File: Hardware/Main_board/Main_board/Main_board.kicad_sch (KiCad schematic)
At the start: 73 parts, among them J2 Conn_01x03_Pin, J3 B9B-XH-A(LF)(SN), J4 282814-2, J5 282814-2, J6 B8B-XH-A(LF)(SN), J6 Power 5V, J7 Power 3v3, J8 GND, J9 Button 1, Q1 2SC1815, U1 L7805, U13 LM358DT, U14 74HC14D, U15 74HC14D, U2 AMS1117-3.3

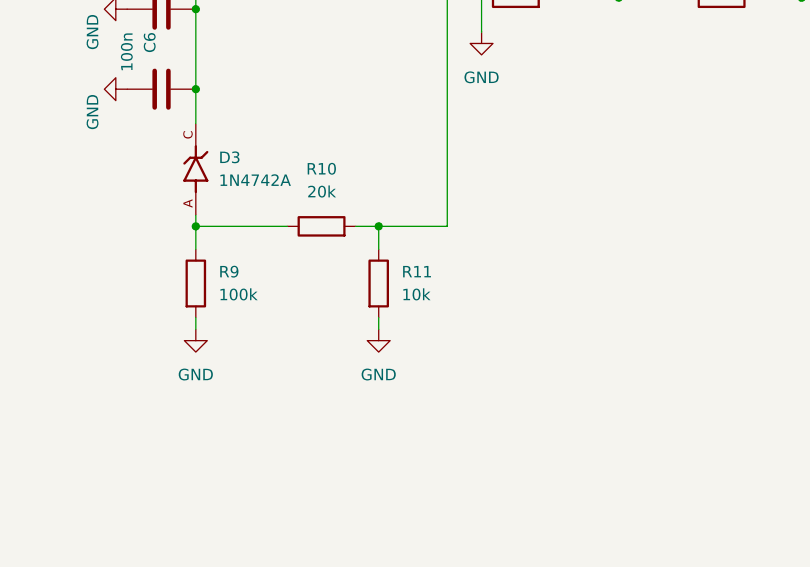
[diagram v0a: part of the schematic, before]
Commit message: after test board
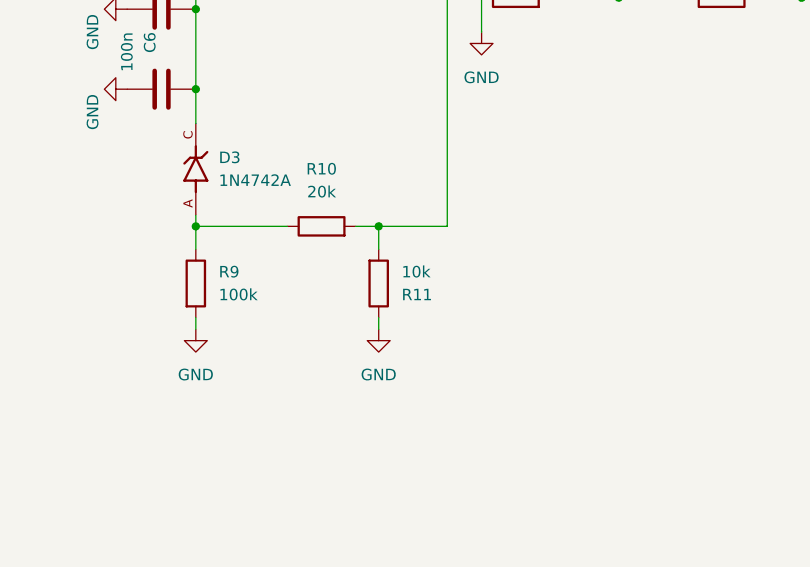
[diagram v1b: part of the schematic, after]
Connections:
- net GND: now also R11.1; no longer R11.2
- net at R10.2, U13.5 (IN2+): now also R11.2; no longer R11.1
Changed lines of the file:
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@@
     )
   )
-  (symbol (lib_id "Device:R") (at 327.66 147.32 0) (unit 1)
-    (in_bom yes) (on_board yes) (dnp no) (fields_autoplaced)
-    (property "Reference" "R11" (at 330.2 146.05 0)
+  (symbol (lib_id "Device:R") (at 327.66 147.32 0) (mirror x) (unit 1)
+    (in_bom yes) (on_board yes) (dnp no)
+    (property "Reference" "R11" (at 330.2 148.59 0)
       (effects (font (size 1.27 1.27)) (justify left))
     )
-    (property "Value" "10k" (at 330.2 148.59 0)
+    (property "Value" "10k" (at 330.2 146.05 0)
       (effects (font (size 1.27 1.27)) (justify left))
     )
